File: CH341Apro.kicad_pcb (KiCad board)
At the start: 2 copper layers, 27.5 x 69 mm, 17 parts, among them J1 USB_A, J3 ZIF-16, J4 , U1 AMS1117-3.3, U2 CH341a, Y1 12M

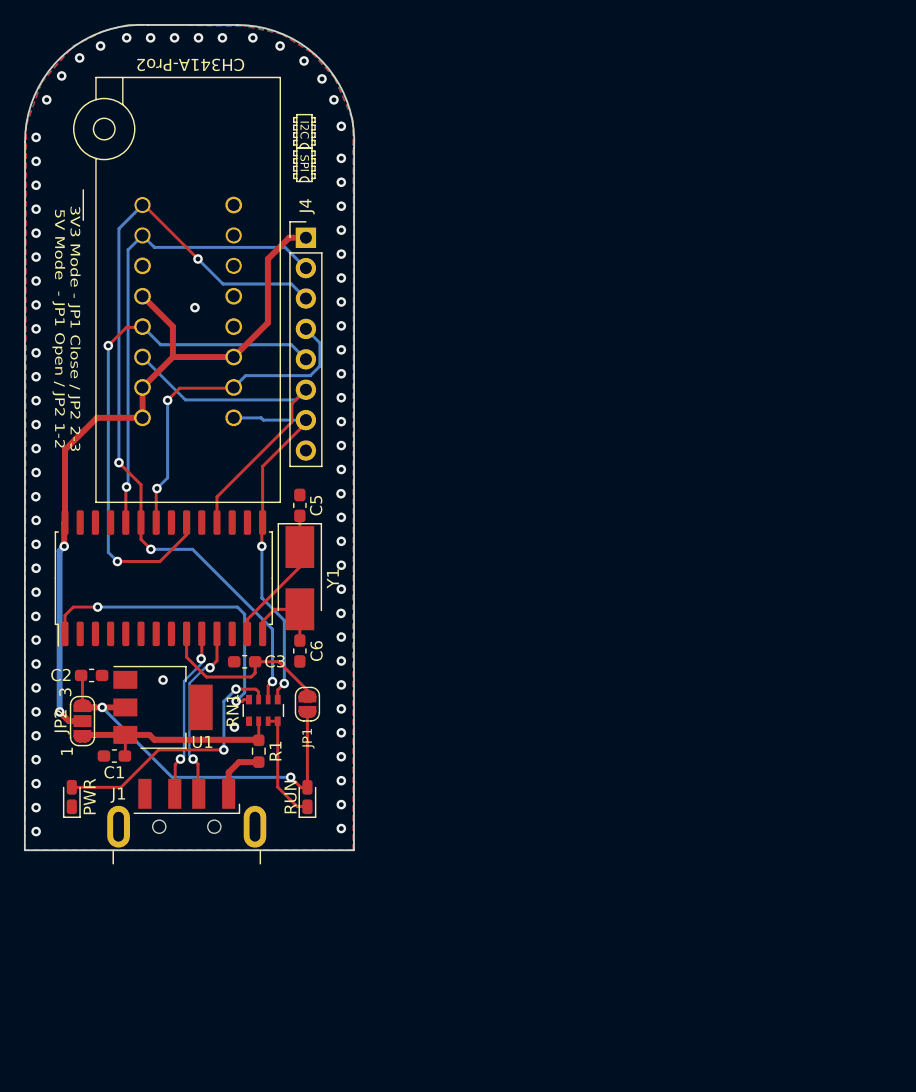
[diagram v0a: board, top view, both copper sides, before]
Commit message: Changed drawing and placement
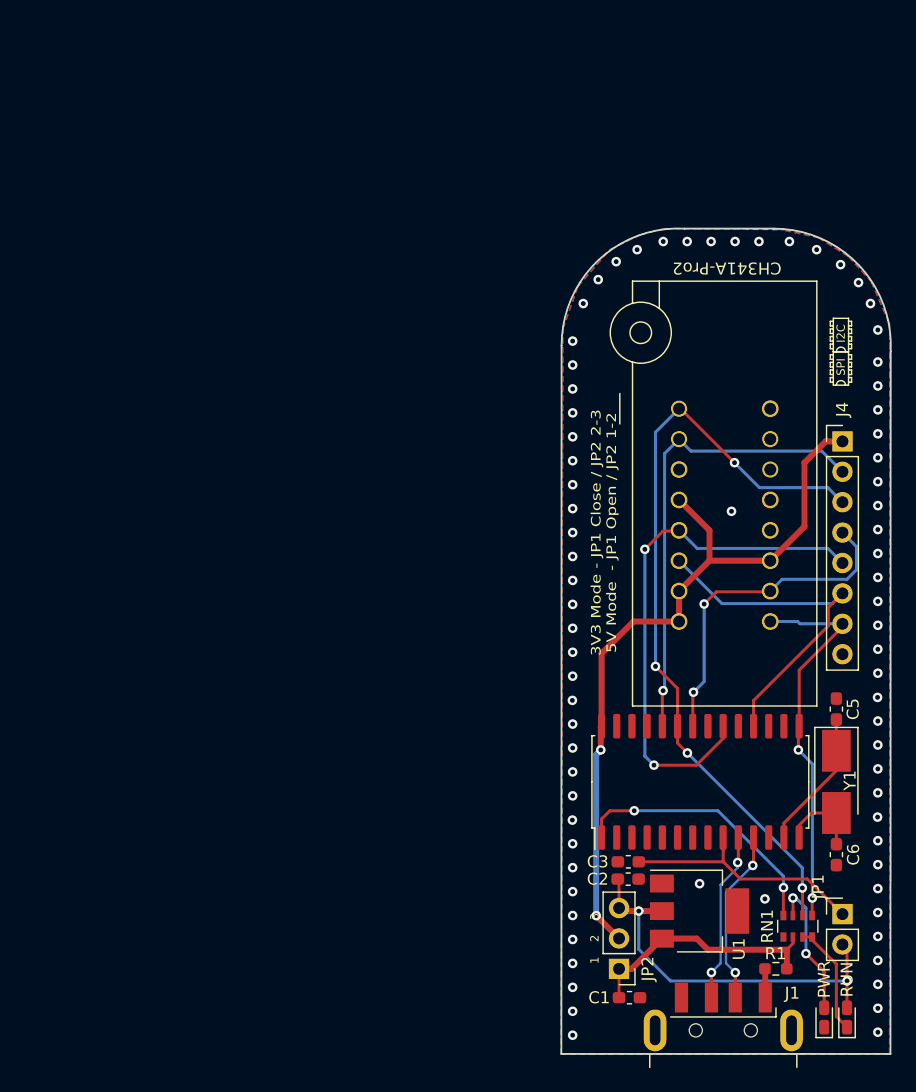
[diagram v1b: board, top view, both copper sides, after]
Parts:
- JP1: footprint Jumper:SolderJumper-2_P1.3mm_Open_RoundedPad1.0x1.5mm -> Connector_PinHeader_2.54mm:PinHeader_1x02_P2.54mm_Vertical
- JP2: footprint Jumper:SolderJumper-3_P1.3mm_Open_RoundedPad1.0x1.5mm_NumberLabels -> Connector_PinHeader_2.54mm:PinHeader_1x03_P2.54mm_Vertical
- moved PWR 65.5 mm to (158.0, 127.9)
- moved JP2 49.4 mm to (140.8, 123.8), turned to 180 degrees
- moved RUN 48.7 mm to (159.9, 127.9)
- moved RN1 48.2 mm to (155.8, 120.3)
- moved JP1 48.0 mm to (159.5, 119.3), turned to 0 degrees
- moved U1 48.0 mm to (147.6, 119.0)
- moved J1 48.0 mm to (149.6, 135.9)
- moved J3 48.0 mm to (145.9, 77.0)
- moved J4 48.0 mm to (159.5, 79.8)
- moved C2 48.0 mm to (141.6, 116.3)
- moved C5 48.0 mm to (159.0, 102.1)
- moved C6 48.0 mm to (159.0, 114.3)
- moved U2 48.0 mm to (147.6, 108.2)
- moved Y1 48.0 mm to (159.0, 108.2)
- moved C1 47.5 mm to (141.7, 126.2), turned to 0 degrees
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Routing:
- net Net-(D1-Pad2): track 22.1 -> 11.9 mm
- net Net-(C3-Pad2): track 15.3 -> 21.9 mm
- net Net-(RN1-Pad4): track 25.8 -> 22.6 mm
- net /5V: track 18.4 -> 20.8 mm
- net Net-(J1-Pad1): track 4.70 -> 2.44 mm
- net /SDA: track 66.5 -> 65.1 mm
- net /3V3: track 32.4 -> 33.2 mm
- net /VCC: track 62.5 -> 63.2 mm
- net /CS: track 32.0 -> 32.5 mm
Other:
- board text added: "1 2 3"
